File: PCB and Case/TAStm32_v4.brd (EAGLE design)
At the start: 50 x 100 mm, 47 parts, among them IC1 74AVCH4T245PW,118, IC2 74AVCH4T245PW,118, IC3 74AVCH4T245PW,118, J1 ZX62D-B-5PA8, J10 RJSSE538002, J11 RJSSE538002, J12 SOICBITE, J13 CONSOLE_RESET, J2 UE27-AC54-100, J3 TSM-105-02-L-SHJ, J4 CONSOLE_RESET, J5 OLED128X64, J6 SAMTEC-TSM-116-01-X-SVJ, J7 SAMTEC-TSM-116-01-X-SVJ, U1 STM32F446RET6, U2 3.3V REG, Y1 8MHz

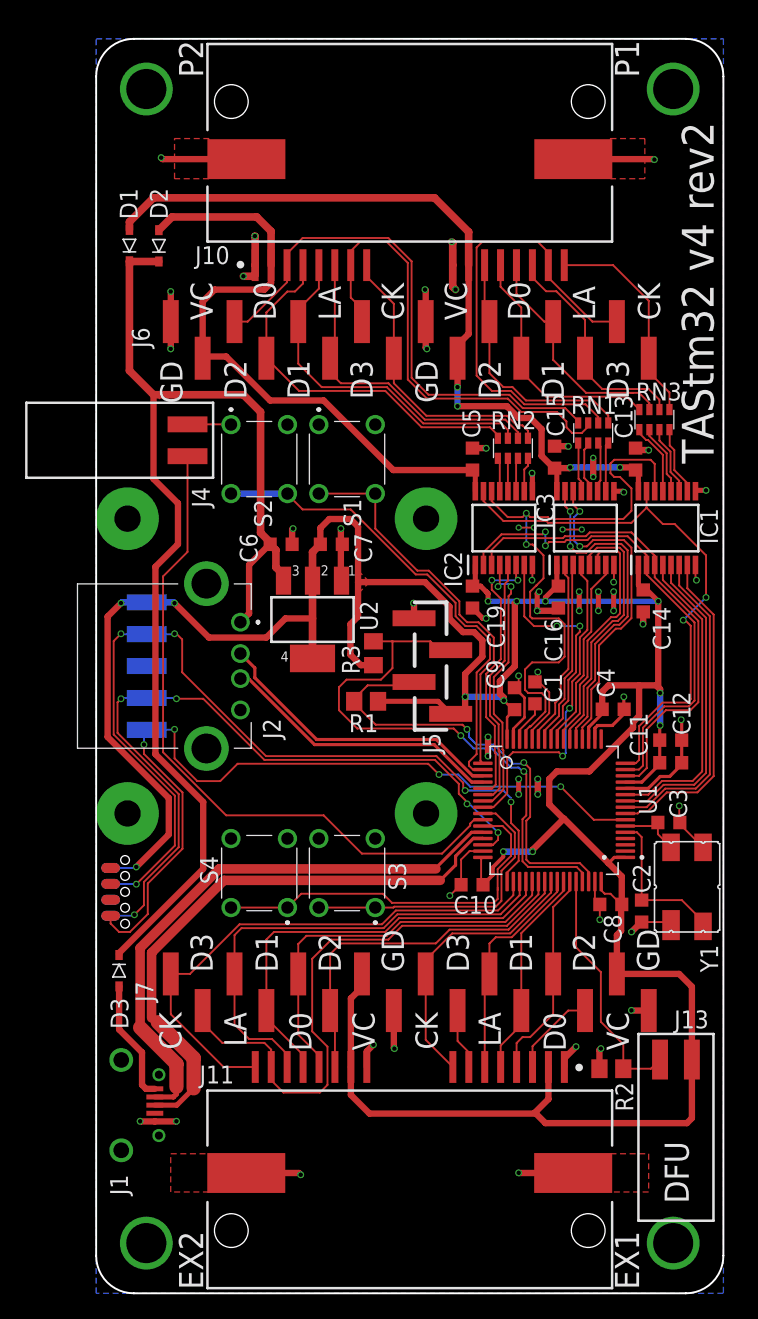
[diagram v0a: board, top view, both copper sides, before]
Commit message: notes
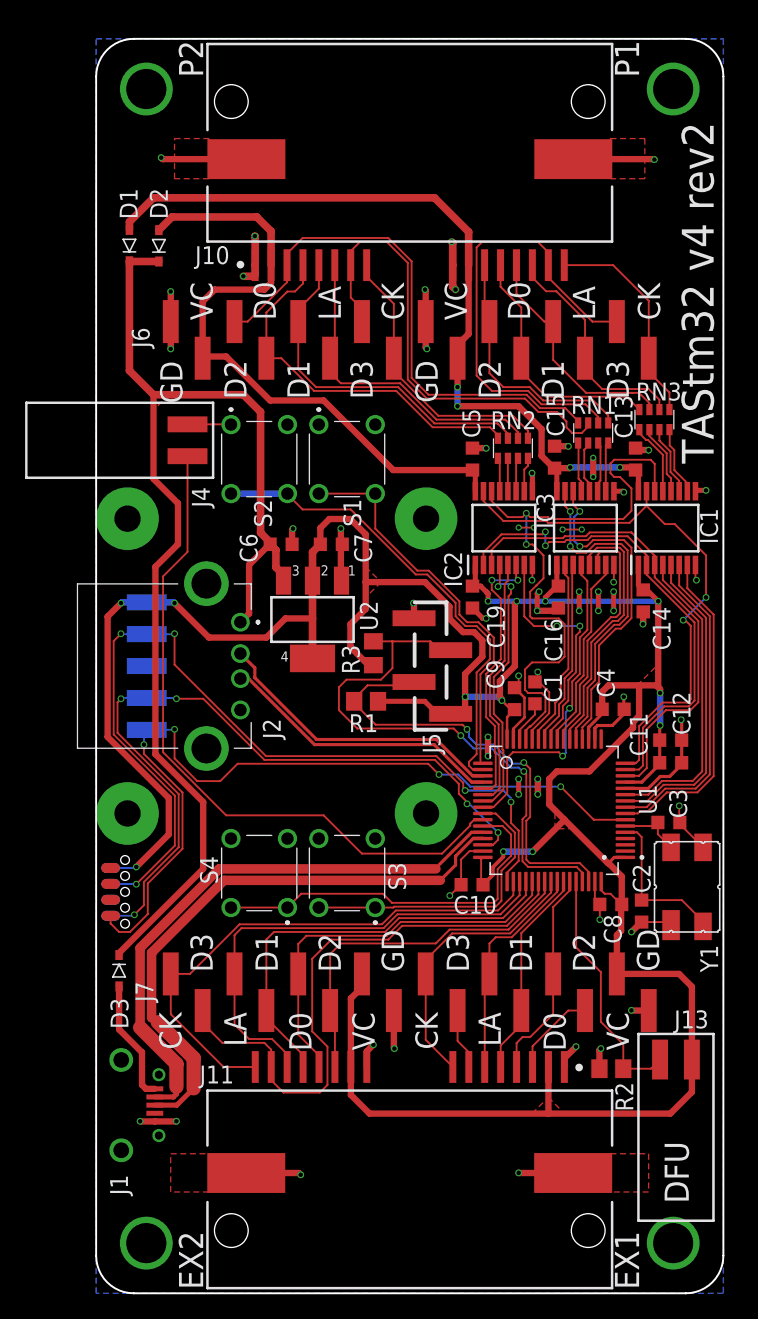
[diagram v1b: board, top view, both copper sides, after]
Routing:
- net V+: track 267.6 -> 264.8 mm
- net P2_CLOCK: track 23.2 -> 22.6 mm
